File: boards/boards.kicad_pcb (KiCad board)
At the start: 2 copper layers, 33 parts, among them J1 MicroSD, P14 CONN_01X01, P15 CONN_01X01, P16 CONN_01X01, P17 CONN_01X01, P18 CONN_01X01, P19 CONN_01X01, P20 CONN_01X01, P21 CONN_01X01, P22 CONN_01X01, U1 LP38690, U2 Teensy_LC, U3 MS5637

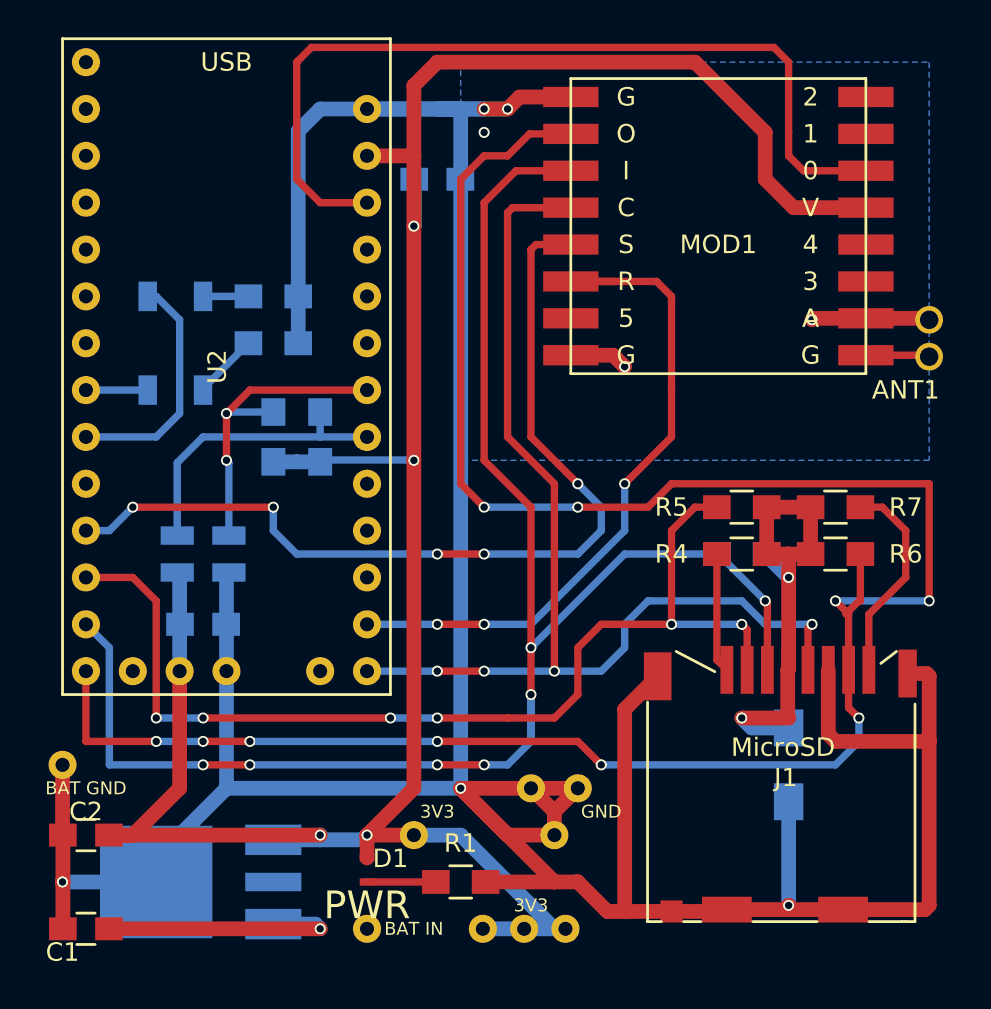
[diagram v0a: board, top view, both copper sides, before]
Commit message: Final modifications to Rev.1 and exported Gerbers.
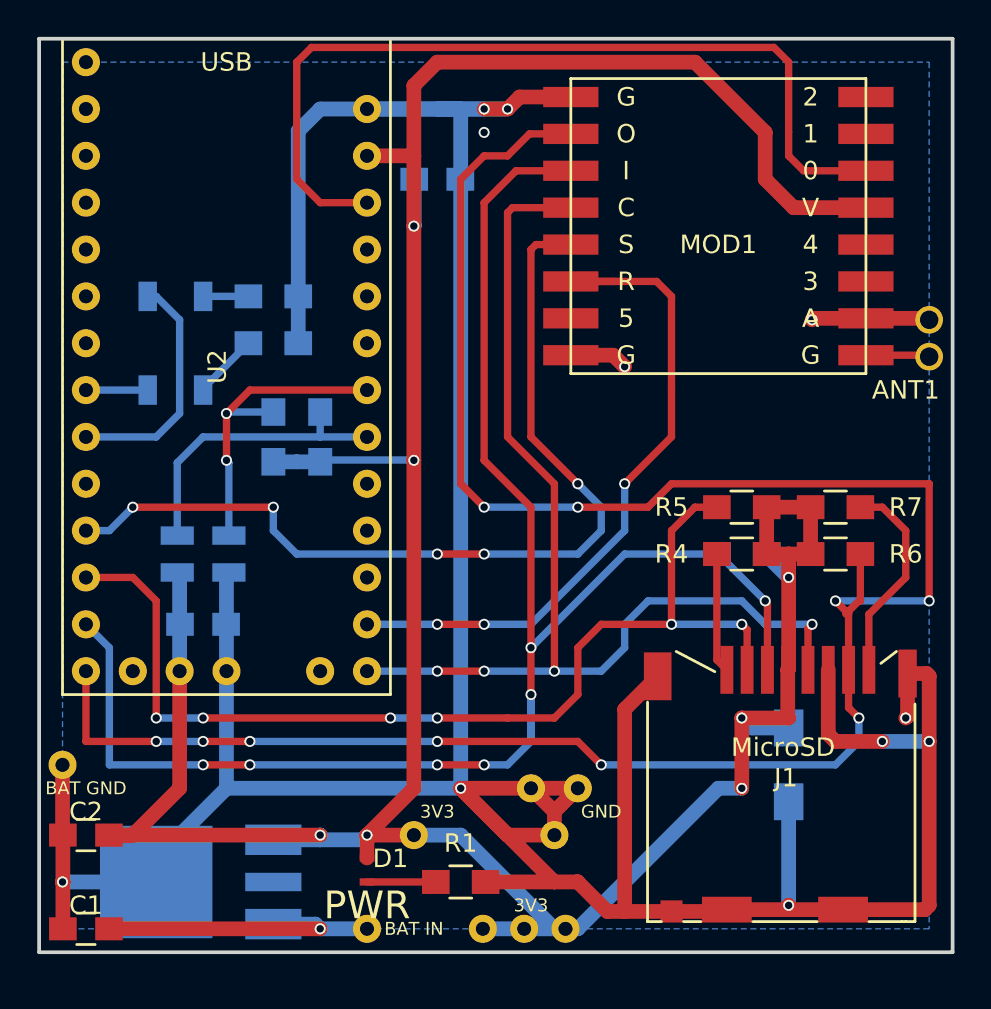
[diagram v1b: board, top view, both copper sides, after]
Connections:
- U1 pad 1: (no net) -> +3V3
- U1 pad 2: (no net) -> GND
- U1 pad 3: (no net) -> VCC
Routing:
- net +3V3: track 164.0 -> 180.5 mm, vias 6 -> 7
- net (no net): track 0.00 -> 3.81 mm
- net VCC: track 14.1 -> 16.6 mm
- net GND: track 219.7 -> 222.2 mm, vias 7 -> 10
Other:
- board outline added: 49.5 x 49.5 mm
- rule pad_to_mask_clearance: 0.2 -> 0
- board text added: "Pickle Rev 1 Telemetry board Designed by W Eustace"
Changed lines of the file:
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@@
 (kicad_pcb (version 4) (host pcbnew 4.0.2-stable)
   (general
-    (links 71)
-    (no_connects 8)
+    (links 74)
+    (no_connects 4)
     (area 43.151667 22.584999 96.620001 74.635)
     (thickness 1.6)
-    (drawings 12)
-    (tracks 330)
+    (drawings 13)
+    (tracks 344)
     (zones 0)
     (modules 33)
@@
     (0 F.Cu signal)
     (31 B.Cu signal)
-    (32 B.Adhes user)
-    (33 F.Adhes user)
-    (34 B.Paste user)
-    (35 F.Paste user)
+    (32 B.Adhes user hide)
+    (33 F.Adhes user hide)
+    (34 B.Paste user hide)
+    (35 F.Paste user hide)
     (36 B.SilkS user)
     (37 F.SilkS user)
-    (38 B.Mask user)
-    (39 F.Mask user)
-    (40 Dwgs.User user)
-    (41 Cmts.User user)
-    (42 Eco1.User user)
-    (43 Eco2.User user)
-    (44 Edge.Cuts user)
-    (45 Margin user)
-    (46 B.CrtYd user)
-    (47 F.CrtYd user)
-    (48 B.Fab user)
-    (49 F.Fab user)
+    (38 B.Mask user hide)
+    (39 F.Mask user hide)
+    (40 Dwgs.User user hide)
+    (41 Cmts.User user hide)
+    (42 Eco1.User user hide)
+    (43 Eco2.User user hide)
+    (44 Edge.Cuts user hide)
+    (45 Margin user hide)
+    (46 B.CrtYd user hide)
+    (47 F.CrtYd user hide)
+    (48 B.Fab user hide)
+    (49 F.Fab user hide)
   )
   (setup
@@
     (trace_min 0.15)
     (segment_width 0.2)
-    (edge_width 0.15)
+    (edge_width 0.2)
     (via_size 0.6)
     (via_drill 0.4)
@@
     (mod_text_size 1 1)
     (mod_text_width 0.15)
-    (pad_size 1.5 1.5)
-    (pad_drill 1)
-    (pad_to_mask_clearance 0.2)
+    (pad_size 6.096 6.096)
+    (pad_drill 0)
+    (pad_to_mask_clearance 0)
     (aux_axis_origin 0 0)
-    (visible_elements FFFEFF7F)
+    (visible_elements FFFEFFFF)
     (pcbplotparams
-      (layerselection 0x00030_80000001)
-      (usegerberextensions false)
+      (layerselection 0x010f0_80000001)
+      (usegerberextensions true)
       (excludeedgelayer true)
       (linewidth 0.100000)
@@
       (outputformat 1)
       (mirror false)
-      (drillshape 1)
+      (drillshape 0)
       (scaleselection 1)
-      (outputdirectory ""))
+      (outputdirectory export/))
   )
   (net 0 "")
@@
     (tags "capacitor 0805")
     (attr smd)
-    (fp_text reference C1 (at 1.27 -1.27 180) (layer F.SilkS)
+    (fp_text reference C1 (at 0 1.27 180) (layer F.SilkS)
       (effects (font (size 1 1) (thickness 0.15)))
     )
@@
     (fp_line (start 3.429 9.398) (end 3.429 7.62) (layer B.SilkS) (width 0.15))
     (pad 4 smd rect (at 0 0 270) (size 1 3.048) (layers B.Cu B.Paste B.Mask))
-    (pad 1 smd rect (at -2.286 0 270) (size 1.651 3.048) (layers B.Cu B.Paste B.Mask))
-    (pad 2 smd rect (at 0 6.35 270) (size 6.096 6.096) (layers B.Cu B.Paste B.Mask))
-    (pad 3 smd rect (at 2.286 0 270) (size 1.651 3.048) (layers B.Cu B.Paste B.Mask))
+    (pad 1 smd rect (at -2.286 0 270) (size 1.651 3.048) (layers B.Cu B.Paste B.Mask)
+      (net 3 +3V3))
+    (pad 2 smd rect (at 0 6.35 270) (size 6.096 6.096) (layers B.Cu B.Paste B.Mask)
+      (net 1 GND))
+    (pad 3 smd rect (at 2.286 0 270) (size 1.651 3.048) (layers B.Cu B.Paste B.Mask)
+      (net 2 VCC))
     (model TO_SOT_Packages_SMD.3dshapes/TO-252-2Lead.wrl
       (at (xyz 0 0 0))
@@
       (net 2 VCC))
   )
+  (gr_text "Pickle Rev 1\nTelemetry board\nDesigned by W Eustace" (at 82.55 33.02) (layer B.SilkS)
+    (effects (font (size 1.5 1.5) (thickness 0.3)) (justify mirror))
+  )
   (gr_text 3V3 (at 73.66 69.85) (layer F.SilkS)
     (effects (font (size 0.7 0.7) (thickness 0.175)))
@@
   )
   (gr_text "SD/GPS OK" (at 54.61 44.45) (layer B.SilkS)
-    (effects (font (size 0.8 0.8) (thickness 0.2)))
+    (effects (font (size 0.8 0.8) (thickness 0.2)) (justify mirror))
   )
   (gr_text RX/TX (at 54.61 34.29) (layer B.SilkS)
-    (effects (font (size 0.8 0.8) (thickness 0.2)))
+    (effects (font (size 0.8 0.8) (thickness 0.2)) (justify mirror))
   )
   (gr_text PWR (at 64.77 69.85) (layer F.SilkS)
     (effects (font (size 1.5 1.5) (thickness 0.3)))
   )
-  (gr_line (start 46.99 72.39) (end 46.99 22.86) (angle 90) (layer B.Fab) (width 0.2))
-  (gr_line (start 96.52 72.39) (end 46.99 72.39) (angle 90) (layer B.Fab) (width 0.2))
-  (gr_line (start 96.52 22.86) (end 96.52 72.39) (angle 90) (layer B.Fab) (width 0.2))
-  (gr_line (start 46.99 22.86) (end 96.52 22.86) (angle 90) (layer B.Fab) (width 0.2))
+  (gr_line (start 46.99 72.39) (end 46.99 22.86) (angle 90) (layer Edge.Cuts) (width 0.2))
+  (gr_line (start 96.52 72.39) (end 46.99 72.39) (angle 90) (layer Edge.Cuts) (width 0.2))
+  (gr_line (start 96.52 22.86) (end 96.52 72.39) (angle 90) (layer Edge.Cuts) (width 0.2))
+  (gr_line (start 46.99 22.86) (end 96.52 22.86) (angle 90) (layer Edge.Cuts) (width 0.2))
+  (segment (start 95.25 62.23) (end 95.25 64.77) (width 0.4) (layer B.Cu) (net 0))
+  (segment (start 95.25 64.77) (end 95.25 66.04) (width 0.4) (layer B.Cu) (net 0))
   (via (at 71.12 27.94) (size 0.6) (drill 0.4) (layers F.Cu B.Cu) (net 0))
+  (segment (start 94.08 57.28) (end 94.08 59.59) (width 0.8) (layer F.Cu) (net 1))
+  (via (at 93.98 59.69) (size 0.6) (drill 0.4) (layers F.Cu B.Cu) (net 1))
+  (segment (start 94.08 59.59) (end 93.98 59.69) (width 0.8) (layer F.Cu) (net 1))
+  (segment (start 90.17 60.96) (end 92.71 60.96) (width 0.8) (layer F.Cu) (net 1))
+  (segment (start 89.78 60.57) (end 90.17 60.96) (width 0.8) (layer F.Cu) (net 1))
+  (segment (start 89.78 57.08) (end 89.78 60.57) (width 0.8) (layer F.Cu) (net 1))
+  (via (at 95.25 60.96) (size 0.6) (drill 0.4) (layers F.Cu B.Cu) (net 1))
+  (segment (start 92.71 60.96) (end 95.25 60.96) (width 0.8) (layer B.Cu) (net 1))
+  (via (at 92.71 60.96) (size 0.6) (drill 0.4) (layers F.Cu B.Cu) (net 1))
   (segment (start 74.93 66.04) (end 74.93 64.77) (width 0.8) (layer F.Cu) (net 1))
   (segment (start 74.93 64.77) (end 73.66 63.5) (width 0.8) (layer F.Cu) (net 1))
@@
   (segment (start 95.25 57.41) (end 95.25 60.96) (width 0.8) (layer F.Cu) (net 1))
   (segment (start 95.12 57.28) (end 95.25 57.41) (width 0.8) (layer F.Cu) (net 1))
-  (segment (start 89.78 57.08) (end 89.78 60.57) (width 0.8) (layer F.Cu) (net 1))
   (segment (start 95.02 70.08) (end 90.58 70.08) (width 0.8) (layer F.Cu) (net 1))
   (segment (start 95.25 69.85) (end 95.02 70.08) (width 0.8) (layer F.Cu) (net 1))
   (segment (start 95.25 60.96) (end 95.25 69.85) (width 0.8) (layer F.Cu) (net 1))
-  (segment (start 90.17 60.96) (end 95.25 60.96) (width 0.8) (layer F.Cu) (net 1))
-  (segment (start 89.78 60.57) (end 90.17 60.96) (width 0.8) (layer F.Cu) (net 1))
   (segment (start 78.74 70.18) (end 78.74 59.22) (width 0.8) (layer F.Cu) (net 1))
   (segment (start 78.74 59.22) (end 80.53 57.43) (width 0.8) (layer F.Cu) (net 1))
@@
   (segment (start 64.77 26.67) (end 71.12 26.67) (width 0.8) (layer B.Cu) (net 1))
   (via (at 71.12 26.67) (size 0.6) (drill 0.4) (layers F.Cu B.Cu) (net 1))
+  (segment (start 64.77 71.12) (end 62.23 71.12) (width 0.8) (layer B.Cu) (net 2))
   (segment (start 50.78 71.12) (end 62.23 71.12) (width 0.8) (layer F.Cu) (net 2))
   (segment (start 61.976 70.866) (end 59.69 70.866) (width 0.8) (layer B.Cu) (net 2))
   (segment (start 62.23 71.12) (end 61.976 70.866) (width 0.8) (layer B.Cu) (net 2))
   (via (at 62.23 71.12) (size 0.6) (drill 0.4) (layers F.Cu B.Cu) (net 2))
+  (segment (start 85.09 63.5) (end 85.09 59.69) (width 0.8) (layer F.Cu) (net 3))
+  (via (at 85.09 63.5) (size 0.6) (drill 0.4) (layers F.Cu B.Cu) (net 3))
+  (segment (start 83.82 63.5) (end 85.09 63.5) (width 0.8) (layer B.Cu) (net 3))
+  (segment (start 76.2 71.12) (end 83.82 63.5) (width 0.8) (layer B.Cu) (net 3))
+  (segment (start 75.53 71.12) (end 76.2 71.12) (width 0.8) (layer B.Cu) (net 3))
   (segment (start 60.96 45.7) (end 67.23 45.7) (width 0.4) (layer B.Cu) (net 3))
   (via (at 67.31 45.72) (size 0.6) (drill 0.4) (layers F.Cu B.Cu) (net 3))
@@
   (segment (start 54.48 49.8) (end 54.48 45.85) (width 0.4) (layer B.Cu) (net 38))
   (zone (net 1) (net_name GND) (layer B.Cu) (hatch edge 0.508)
-    (connect_pads (clearance 0.508))
+    (connect_pads yes (clearance 0.508))
     (min_thickness 0.254)
     (fill yes (arc_segments 16) (thermal_gap 0.508) (thermal_bridge_width 0.508))
     (polygon
       (pts
-        (xy 69.85 24.13) (xy 95.25 24.13) (xy 95.25 45.72) (xy 69.85 45.72)
+        (xy 48.26 24.13) (xy 95.25 24.13) (xy 95.25 71.12) (xy 48.26 71.12)
       )
     )
